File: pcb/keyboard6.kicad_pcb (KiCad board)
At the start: 2 copper layers, 149.9 x 129.4 mm, 80 parts, among them J1 AudioJack4, J2 USB_B_Micro, SW1 SW_DIP_x01, SW10 SW_DIP_x01, SW11 SW_DIP_x01, SW12 SW_DIP_x01, SW13 SW_DIP_x01, SW14 SW_DIP_x01, SW15 SW_DIP_x01, SW16 SW_DIP_x01, SW17 SW_DIP_x01, SW18 SW_DIP_x01, SW19 SW_DIP_x01, SW2 SW_DIP_x01, SW20 SW_DIP_x01, SW21 SW_DIP_x01, SW22 SW_DIP_x01, SW23 SW_DIP_x01, SW24 SW_DIP_x01, SW25 SW_DIP_x01, SW26 SW_DIP_x01, SW27 SW_DIP_x01, SW28 SW_DIP_x01, SW29 SW_DIP_x01, SW3 SW_DIP_x01, SW30 SW_Push_Dual, SW4 SW_DIP_x01, SW5 SW_DIP_x01, SW6 SW_DIP_x01, SW7 SW_DIP_x01, SW8 SW_DIP_x01, SW9 SW_DIP_x01, Y1 16MHz

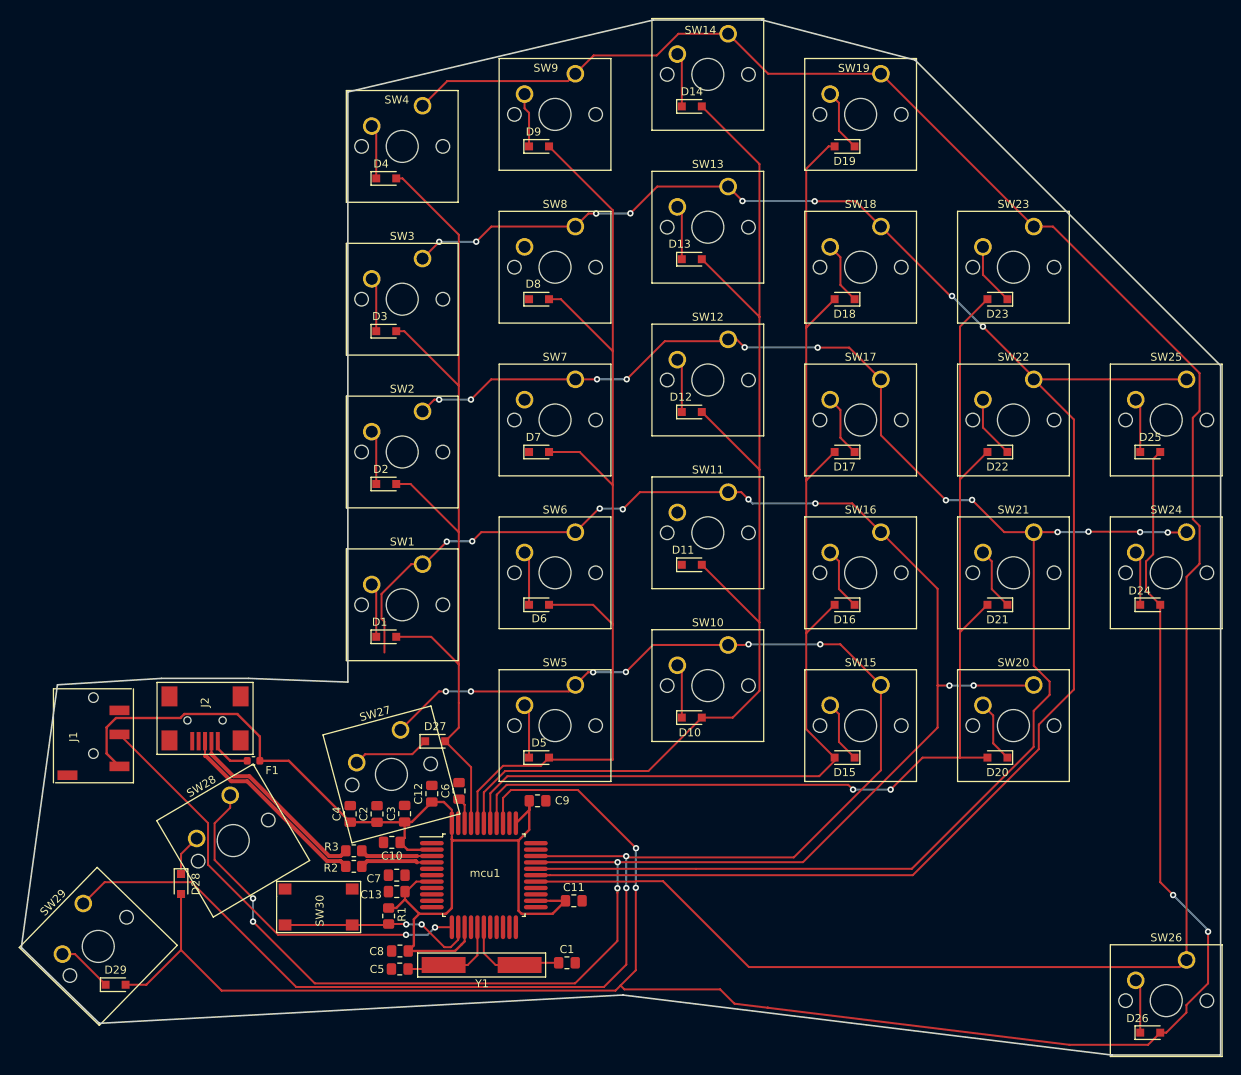
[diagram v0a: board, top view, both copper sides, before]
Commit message: minor change.
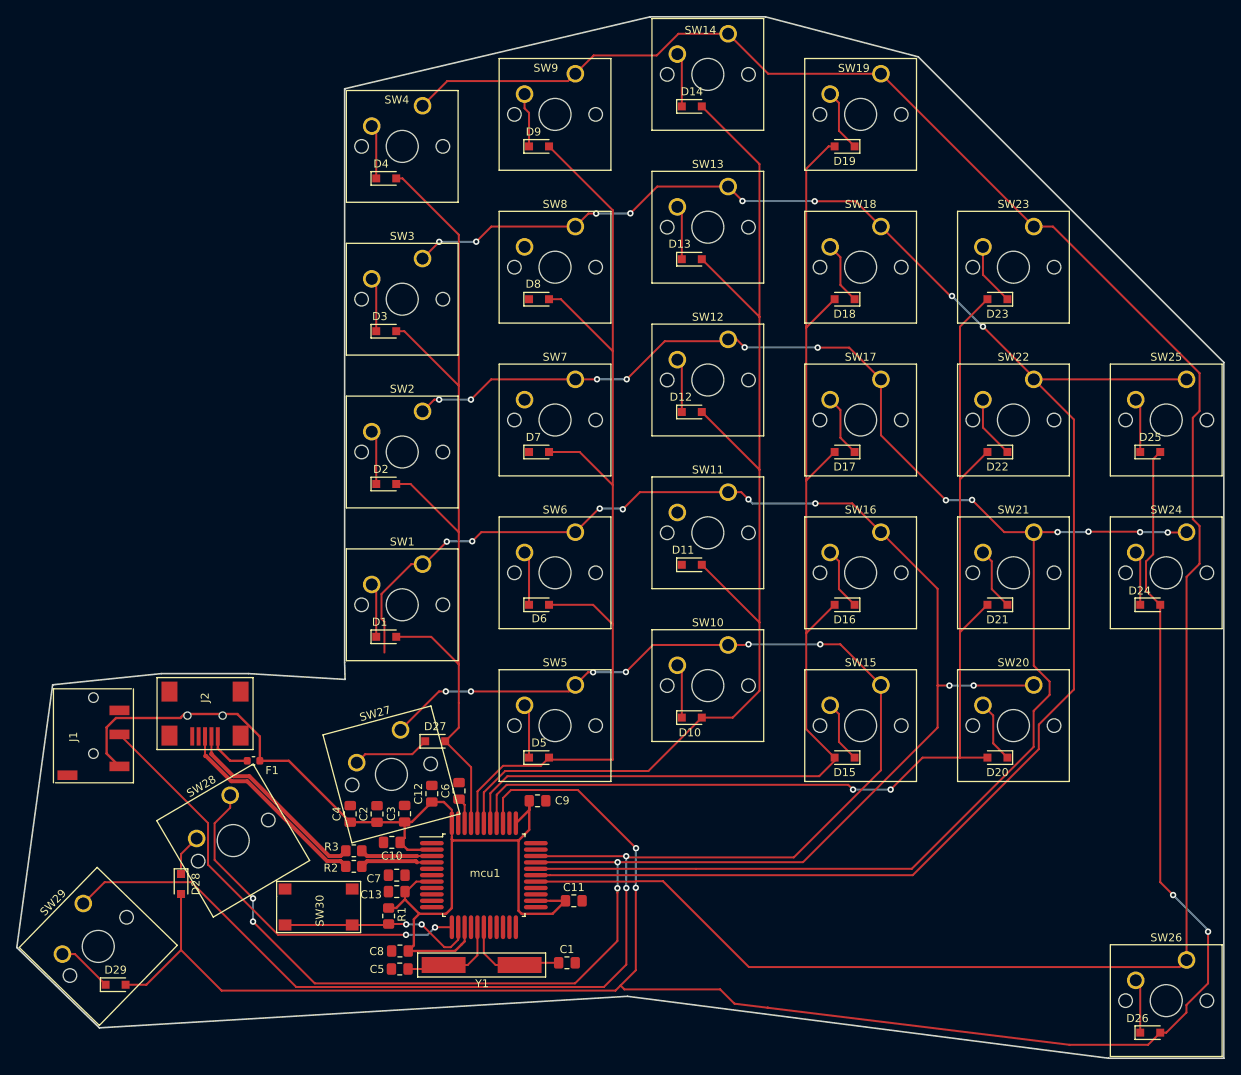
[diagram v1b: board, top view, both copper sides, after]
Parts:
- moved J2 0.60 mm to (-24.6, -10.5)
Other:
- board size 149.9 x 129.4 mm -> 150.9 x 130.2 mm
